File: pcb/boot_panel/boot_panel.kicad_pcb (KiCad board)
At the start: 2 copper layers, 110 x 36 mm, 17 parts, among them J2 Conn_01x06_Pin, U4 AT42QT1070-S

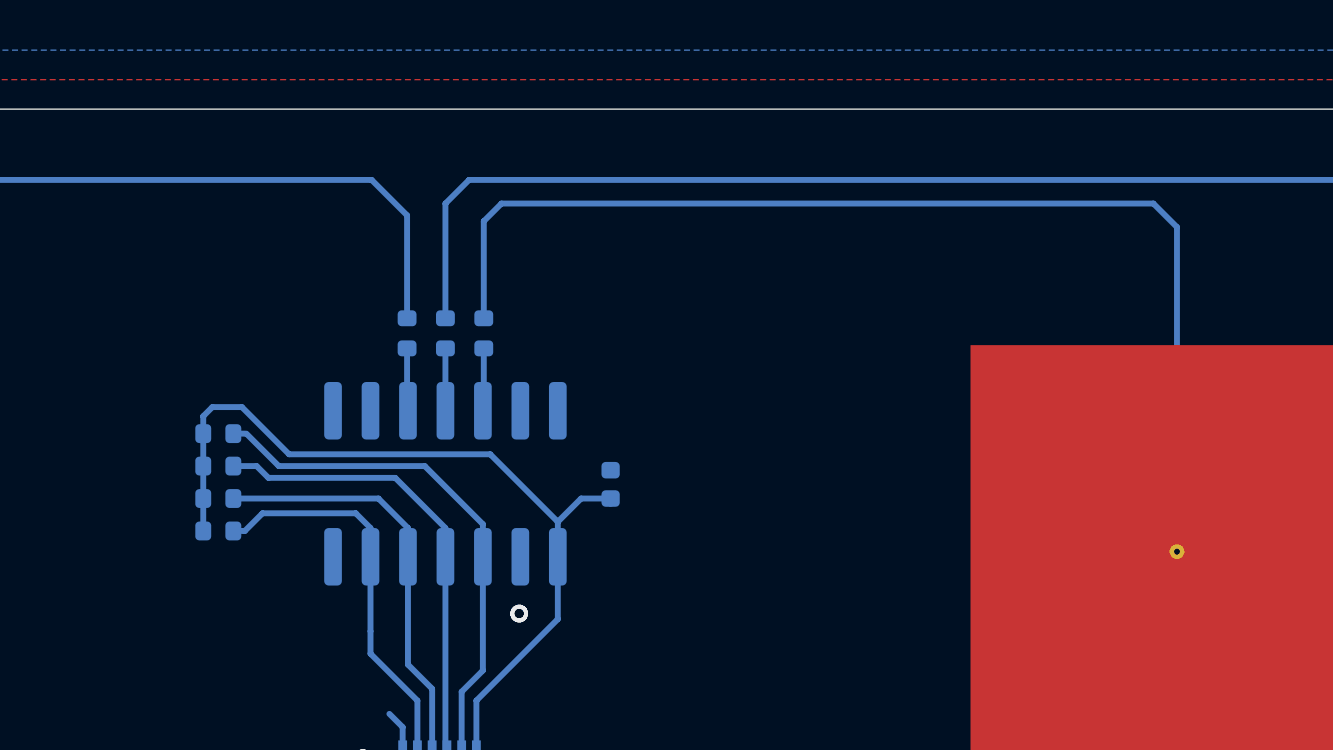
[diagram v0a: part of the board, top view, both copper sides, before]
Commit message: More layout
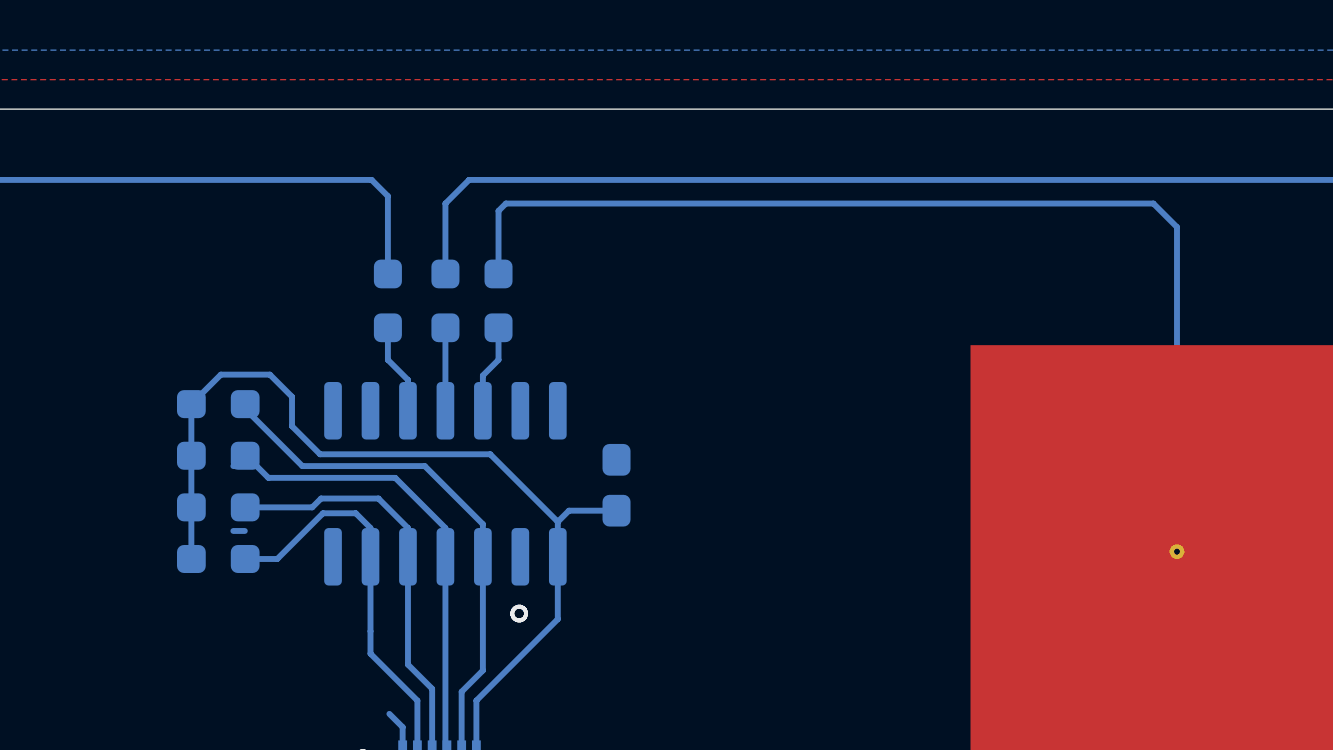
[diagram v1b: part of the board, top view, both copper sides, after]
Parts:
- C1: footprint Capacitor_SMD:C_0402_1005Metric -> Capacitor_SMD:C_0603_1608Metric_Pad1.08x0.95mm_HandSolder
- R1, R2, R3, R4, R5, R6, R7: footprint Resistor_SMD:R_0402_1005Metric -> Resistor_SMD:R_0603_1608Metric_Pad0.98x0.95mm_HandSolder
- moved R4 1.28 mm to (140.2, 70.5)
- moved R2 1.21 mm to (144.0, 70.5)
- moved R3 1.10 mm to (142.2, 70.5)
- moved R1 1.00 mm to (134.5, 74.0)
- moved R5 0.95 mm to (134.5, 79.2)
- moved R6 0.35 mm to (134.5, 75.8)
- moved R7 0.30 mm to (134.5, 77.5)
- moved C1 0.20 mm to (148.0, 76.8)
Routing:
- net +3V3: track 29.2 -> 32.1 mm
- net Net-(U2-PAD): track 37.8 -> 36.0 mm
- net Net-(U1-PAD): track 38.4 -> 36.6 mm
- net Net-(U3-PAD): track 65.1 -> 63.6 mm
- net Net-(U4-KEY3): track 2.13 -> 3.14 mm
- net Net-(U4-KEY1): track 2.13 -> 3.07 mm
- net Net-(U4-KEY2): track 2.11 -> 2.81 mm
